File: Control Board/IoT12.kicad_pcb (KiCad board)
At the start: 2 copper layers, 99.1 x 69.8 mm, 110 parts, among them J10 USB_B_Micro, J11 Conn_ARM_JTAG_SWD_10, J9 Conn_ARM_JTAG_SWD_10, Q1 MMBT2222, Q2 MMBT2222, Q3 AOD403, SW1 Rotary encoder EC11 Plum 15mm, SW2 SW_Push, U1 ATSAMD21G18A-AU, U2 ADS1115IDGS, U3 INA826AID, U4 INA826AID, U5 LM2596S-ADJ, U6 AT24C32, Y1 32768Hz

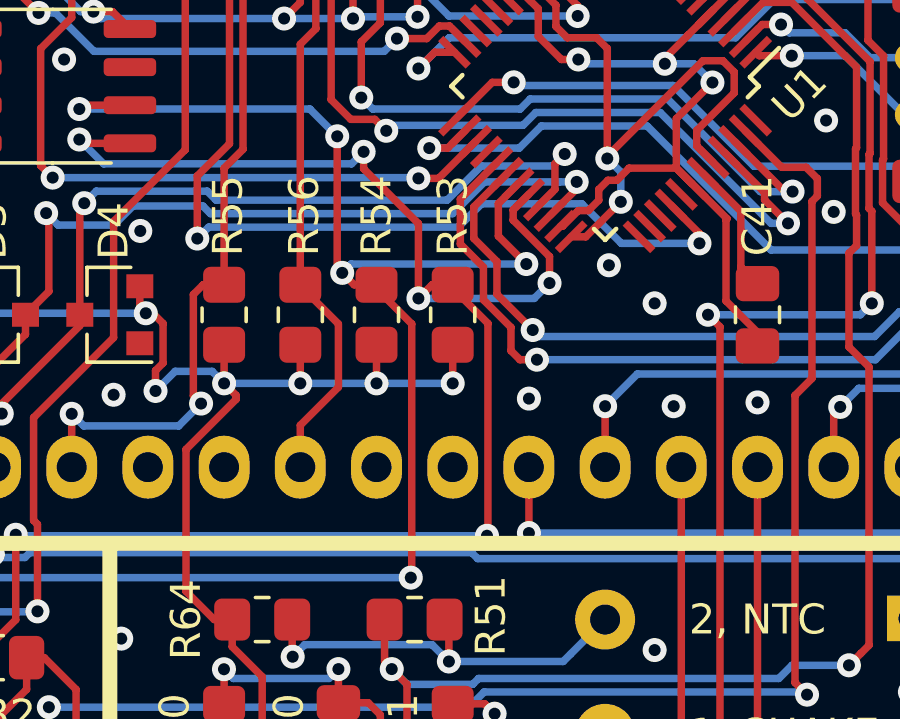
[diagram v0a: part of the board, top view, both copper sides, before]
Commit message: More erratum.
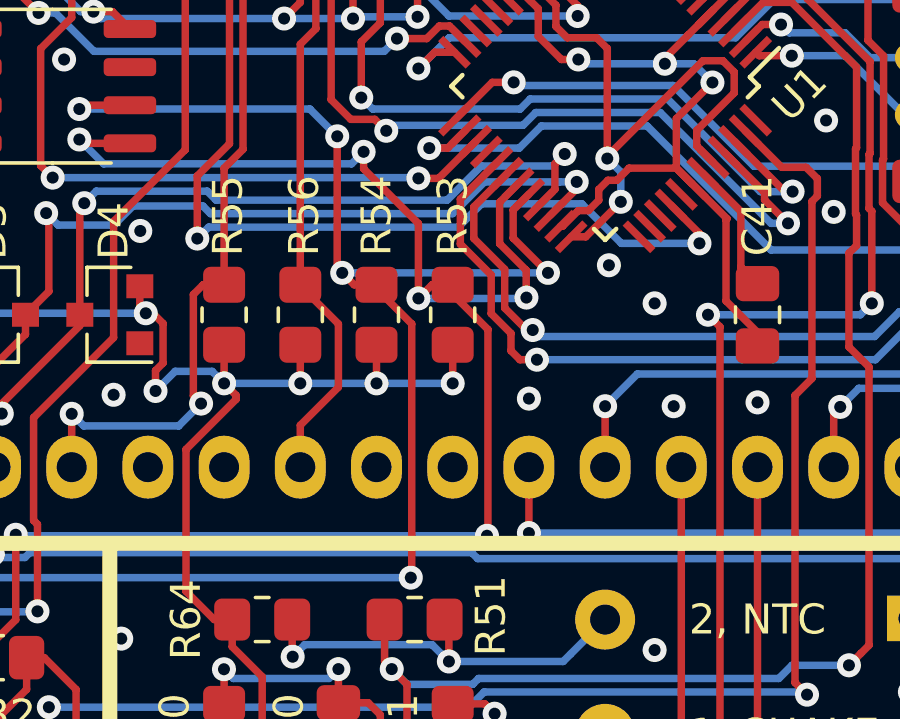
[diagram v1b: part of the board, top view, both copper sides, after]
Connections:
- U1 pad 31: HEAT_SCL -> HEAT_SDA
- U1 pad 32: HEAT_SDA -> HEAT_SCL
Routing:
- net HEAT_SCL: track 58.6 -> 59.2 mm
